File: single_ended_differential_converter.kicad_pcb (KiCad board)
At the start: 2 copper layers, 63.5 x 67.3 mm, 27 parts, among them J1 Conn_Coaxial, J2 Conn_Coaxial, J5 XLR3, U1 PWR_JACK_POS, U2 PWR_JACK_GND, U3 PWR_JACK_NEG, U4 ADA4941-1

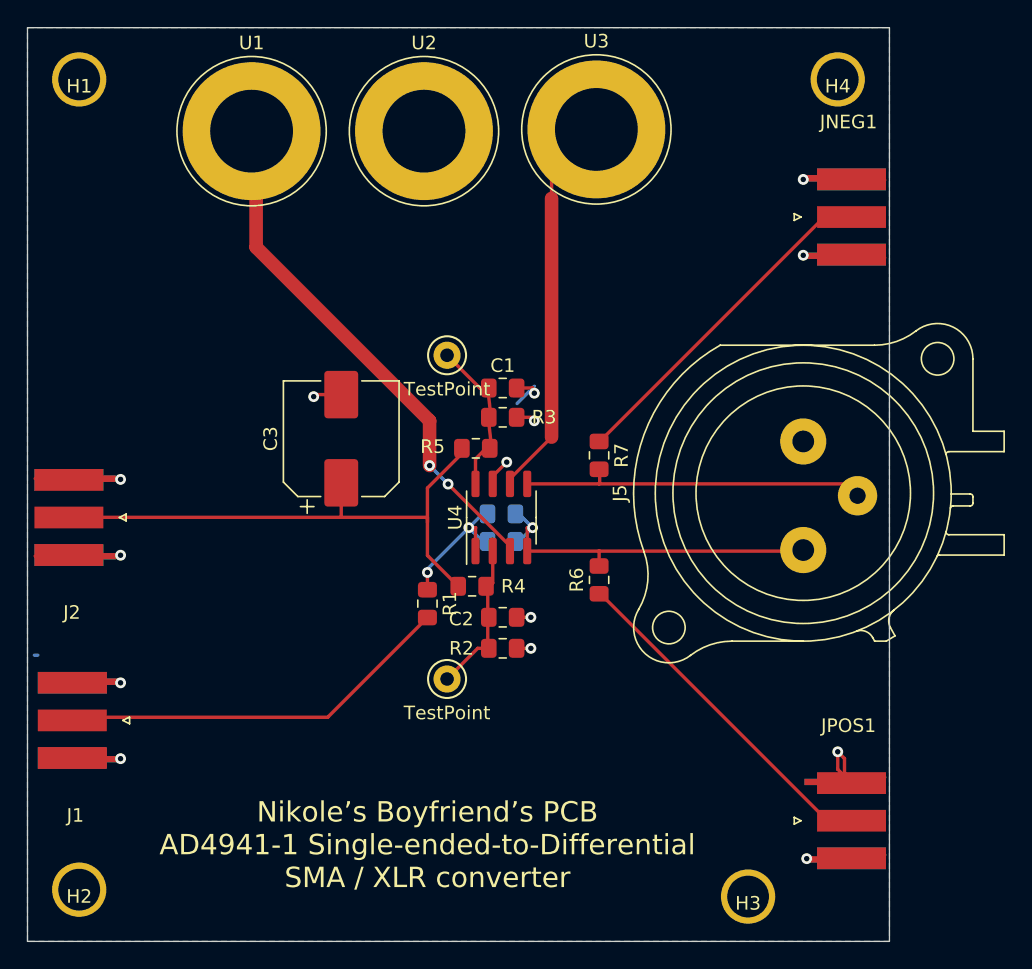
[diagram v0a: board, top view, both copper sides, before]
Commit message: added files for version 2
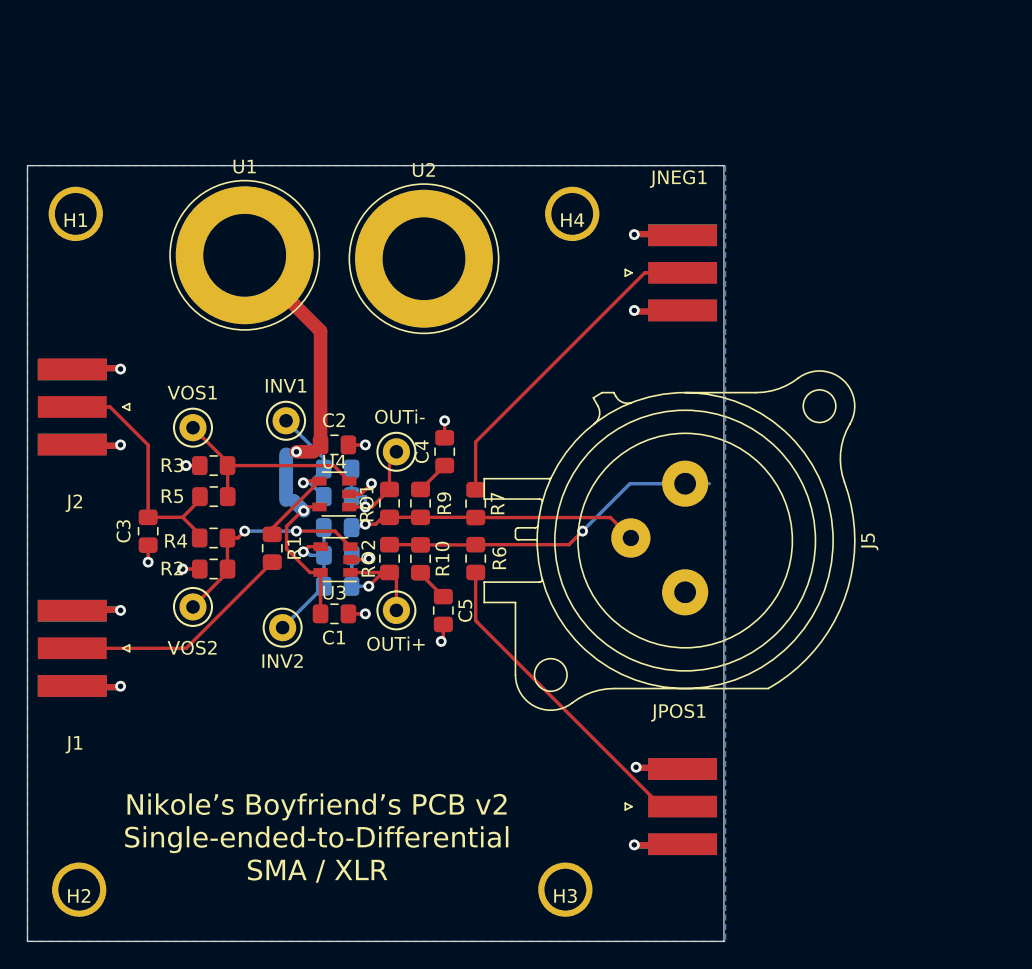
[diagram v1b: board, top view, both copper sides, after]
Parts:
- added C4: C, Capacitor_SMD:C_0805_2012Metric_Pad1.15x1.40mm_HandSolder, F.Cu at (242.8, 127.8)
- added C5: C, Capacitor_SMD:C_0805_2012Metric_Pad1.15x1.40mm_HandSolder, F.Cu at (242.7, 139.5)
- added CF2: 100pF, Capacitor_SMD:C_0805_2012Metric_Pad1.15x1.40mm_HandSolder, B.Cu at (235.0, 135.4)
- added R10: R_US, Resistor_SMD:R_0805_2012Metric_Pad1.15x1.40mm_HandSolder, F.Cu at (241.0, 135.6)
- added R8: 10k, Resistor_SMD:R_0805_2012Metric_Pad1.15x1.40mm_HandSolder, B.Cu at (234.9, 133.3)
- added R9: R_US, Resistor_SMD:R_0805_2012Metric_Pad1.15x1.40mm_HandSolder, F.Cu at (241.0, 131.6)
- added RF2: 10k, Resistor_SMD:R_0805_2012Metric_Pad1.15x1.40mm_HandSolder, B.Cu at (234.9, 137.7)
- added RO1: R_US, Resistor_SMD:R_0805_2012Metric_Pad1.15x1.40mm_HandSolder, F.Cu at (238.8, 131.6)
- added RO2: R_US, Resistor_SMD:R_0805_2012Metric_Pad1.15x1.40mm_HandSolder, F.Cu at (238.8, 135.6)
- added TP1: OUTi-, my_library_foot:TestPoint_Keystone_5000-5004_Miniature, F.Cu at (239.3, 127.8)
- added TP2: OUTi+, my_library_foot:TestPoint_Keystone_5000-5004_Miniature, F.Cu at (239.3, 139.4)
- added TP3: INV1, my_library_foot:TestPoint_Keystone_5000-5004_Miniature, F.Cu at (231.1, 125.5)
- added TP4: INV2, my_library_foot:TestPoint_Keystone_5000-5004_Miniature, F.Cu at (230.9, 140.7)
- C3: value 100uF -> 10uF; footprint Capacitor_SMD:CP_Elec_8x10 -> Capacitor_SMD:C_0805_2012Metric_Pad1.15x1.40mm_HandSolder
- CF1: value ? -> 100pF
- R1, R2, R3, R4, RF1: value R_US -> 10k
- R5: value R_US -> 30k
- U3: value PWR_JACK_NEG -> OPA376xxDBV; footprint Connector:Banana_Jack_1Pin -> Package_TO_SOT_SMD:SOT-23-5
- U4: value ADA4941-1 -> OPA376xxDBV; footprint Package_SO:SOIC-8_3.9x4.9mm_P1.27mm -> Package_TO_SOT_SMD:SOT-23-5
- VOS1: value TestPoint -> VOS1
- VOS2: value TestPoint -> VOS2
- moved U3 33.1 mm to (234.7, 130.9), turned to 180 degrees
- moved R2 22.1 mm to (225.8, 136.4), turned to 180 degrees
- moved H4 21.9 mm to (252.2, 110.2)
- moved R3 21.6 mm to (225.8, 128.8), turned to 180 degrees
- moved C1 20.7 mm to (234.7, 139.7)
- moved R5 19.6 mm to (225.8, 131.1)
- moved VOS2 19.5 mm to (224.3, 126.0)
- moved VOS1 19.5 mm to (224.3, 139.2)
- moved R4 19.4 mm to (225.8, 134.1)
- moved C2 17.7 mm to (234.7, 127.3)
- moved C3 15.8 mm to (221.0, 133.6), turned to 270 degrees
- moved J5 14.1 mm to (260.5, 138.1), turned to 270 degrees
- moved H3 13.5 mm to (251.7, 160.0)
- moved CF1 13.2 mm to (234.9, 129.0)
- moved JNEG1 13.1 mm to (258.6, 114.6)
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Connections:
- C1 pad 1: /VOS2 -> VDD
- C2 pad 1: /VOS1 -> VDD
- CF1 pad 1: /VoutP -> /OUTi-
- CF1 pad 2: Net-(CF1-Pad2) -> /INV1
- J5 pad 2: /VoutP -> /OUT+
- J5 pad 3: /VoutN -> /OUT-
- R1 pad 1: Net-(CF1-Pad2) -> /INV1
- R2 pad 1: /VOS1 -> /VOS2
- R3 pad 1: /VOS2 -> /VOS1
- R4 pad 2: /VOS1 -> /VOS2
- R5 pad 2: /VOS2 -> /VOS1
- R6 pad 2: /VoutP -> /OUT+
- R7 pad 2: /VoutN -> /OUT-
- RF1 pad 1: /VoutP -> /OUTi-
- RF1 pad 2: Net-(CF1-Pad2) -> /INV1
- U3 pad 1: VSS -> /OUTi-
- U4 pad 1: Net-(CF1-Pad2) -> /OUTi+
- U4 pad 2: /VOS1 -> GND
- U4 pad 3: VDD -> /VOS2
- U4 pad 4: /VoutP -> /INV2
- U4 pad 5: /VoutN -> VDD
- VOS1 pad 1: /VOS1 -> /VOS2
- VOS2 pad 1: /VOS2 -> /VOS1
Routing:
- net VSS: track 27.8 -> 0.00 mm
- net /OUT+: track 0.00 -> 27.0 mm, vias 0 -> 1
- net /VoutP: track 26.5 -> 0.00 mm, vias 1 -> 0
- net /VoutN: track 25.9 -> 0.00 mm
- net GND: track 68.3 -> 43.7 mm, vias 14 -> 17
- net /Vref: track 40.6 -> 18.7 mm
- net /OUT-: track 0.00 -> 21.0 mm, vias 0 -> 1
- net /INV1: track 0.00 -> 14.7 mm, vias 0 -> 1
- net Net-(CF1-Pad2): track 11.8 -> 0.00 mm, vias 2 -> 0
- net /Vin: track 29.1 -> 17.4 mm
- net /INV2: track 0.00 -> 11.7 mm, vias 0 -> 1
- net /OUTi-: track 0.00 -> 10.7 mm, vias 0 -> 1
- net /OUTi+: track 0.00 -> 10.4 mm, vias 0 -> 1
- net VDD: track 40.9 -> 35.4 mm
- net /VOS2: track 11.9 -> 15.9 mm, vias 0 -> 2
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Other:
- board size 63.5 x 67.3 mm -> 51.3 x 57.2 mm
- board text added: "Nikole’s Boyfriend’s PCB v2 Single-ended-to-Differential SMA / XLR"
- board text removed: "Nikole’s Boyfriend’s PCB AD4941-1 Single-ended-to-Differential SMA / XLR converter"
